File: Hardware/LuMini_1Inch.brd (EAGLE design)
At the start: 28.7 x 43.2 mm, 48 parts, among them J1 SOLDER_PAD_2, J2 SOLDER_PAD_2, J4 SOLDER_PAD_2

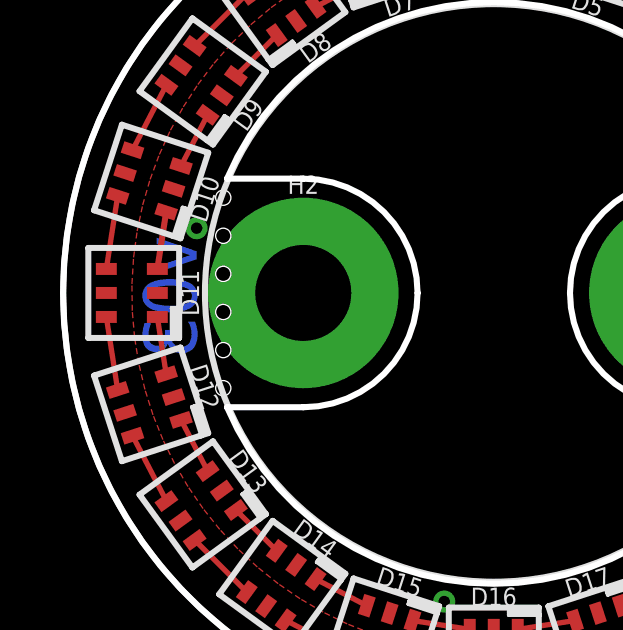
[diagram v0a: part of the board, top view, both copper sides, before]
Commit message: version number change
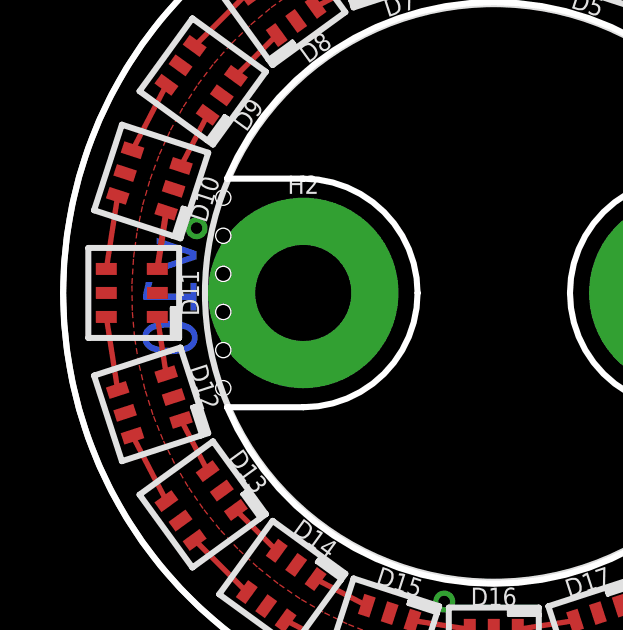
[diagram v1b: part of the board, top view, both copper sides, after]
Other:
- board text added: "v10"
- board text removed: "v03"
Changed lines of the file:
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@@
 <plain>
 <circle x="14.605" y="21.59" radius="14.351" width="0.2032" layer="21"/>
-<text x="4.699" y="23.495" size="1.778" layer="16" font="vector" ratio="15" rot="SMR270">v03</text>
+<text x="4.699" y="23.495" size="1.778" layer="16" font="vector" ratio="15" rot="SMR270">v10</text>
 <hole x="5.588" y="18.415" drill="0.508"/>
 <wire x1="5.715" y1="17.78" x2="8.255" y2="17.78" width="0.2032" layer="20"/>
